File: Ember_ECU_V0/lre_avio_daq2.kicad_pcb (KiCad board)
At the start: 4 copper layers, 13.4 x 4.5 mm, 172 parts, among them J1 Conn_01x02_Socket, J10 Conn_01x02_Pin, J11 USB_C_Receptacle_USB2.0_16P, J12 XT30PW-F, J13 XT30PW-F, J14 XT30PW-F, J15 XT30PW-F, J16 XT30PW-F, J17 SMPW-CC-K-M, J18 SMPW-CC-K-M, J19 SMPW-CC-K-M, J2 DB25_Socket_MountingHoles, J20 Conn_01x02_Pin, J23 DA15_Socket_MountingHoles, J24 DB25_Socket_MountingHoles, J3 XT60PW-M, J4 Conn_01x02_Socket, Q1 SISA96DN-T1-GE3, Q2 SISA96DN-T1-GE3, Q3 SISA96DN-T1-GE3, SW1 SW_SPDT, U1 AMS1117-5.0, U10 ADS8353QPWRQ1, U11 ADS8353QPWRQ1, U12 STM32F412VGTx, U13 HX711, U14 HX711, U15 WS2812B-2020, U16 WS2812B-2020, U17 WS2812B-2020, U18 TCAN330, U2 HX711, U4 HX711, U5 AMS1117-5.0, U6 ADS8353QPWRQ1, U7 MAX31856, U8 MAX31856, U9 MAX31856, Y1 Crystal_8Mhz

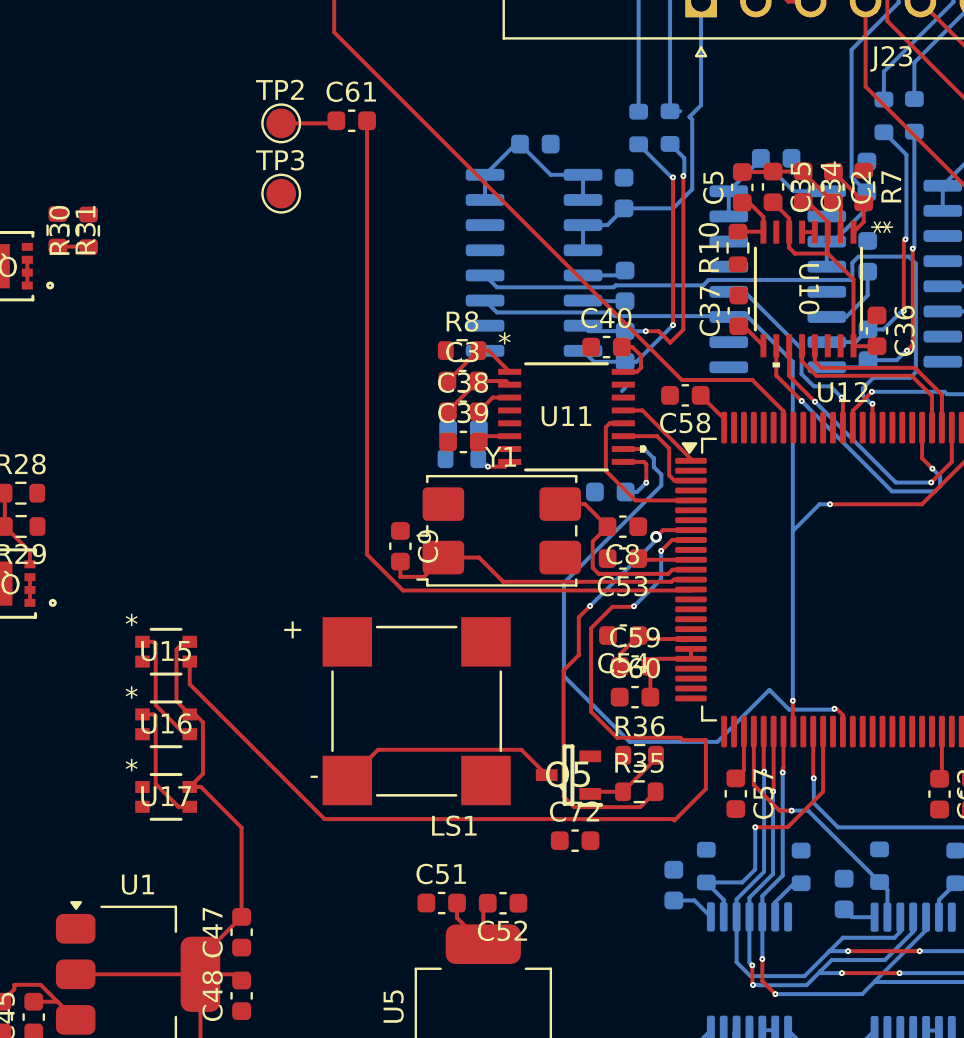
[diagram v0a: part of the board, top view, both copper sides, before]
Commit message: partial schematics fixes
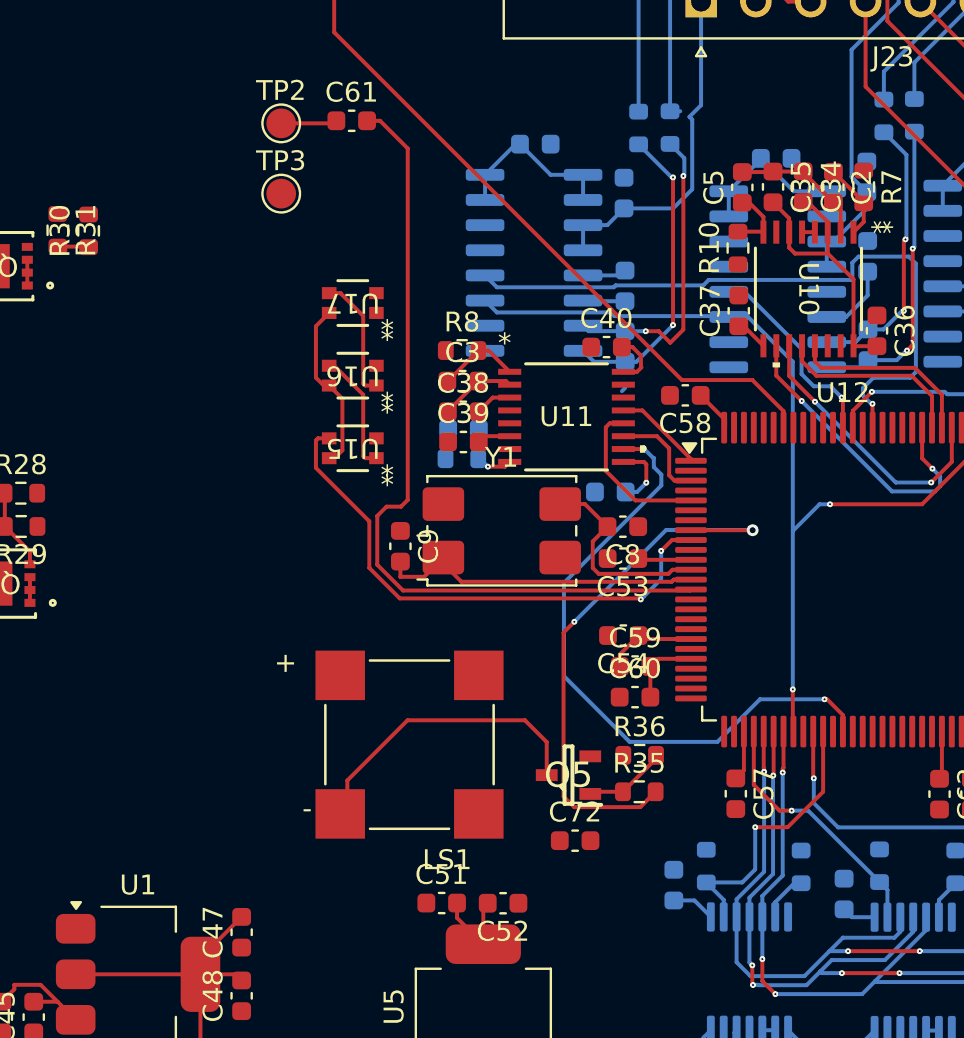
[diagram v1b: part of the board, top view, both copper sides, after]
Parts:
- moved U17 26.7 mm to (189.7, 65.6), turned to 180 degrees
- moved U16 20.0 mm to (189.7, 69.3), turned to 180 degrees
- moved U15 13.9 mm to (189.7, 72.9), turned to 180 degrees
- moved LS1 1.73 mm to (192.5, 87.9)
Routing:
- net /DI1: track 51.5 -> 27.3 mm
- net /5v: track 89.3 -> 81.3 mm
- net /Buzzer_G: track 22.2 -> 28.5 mm
- net Net-(Q5-D): track 11.2 -> 15.4 mm
- net Net-(U12-NRST): track 39.0 -> 41.1 mm
- net GND: track 36.2 -> 35.7 mm

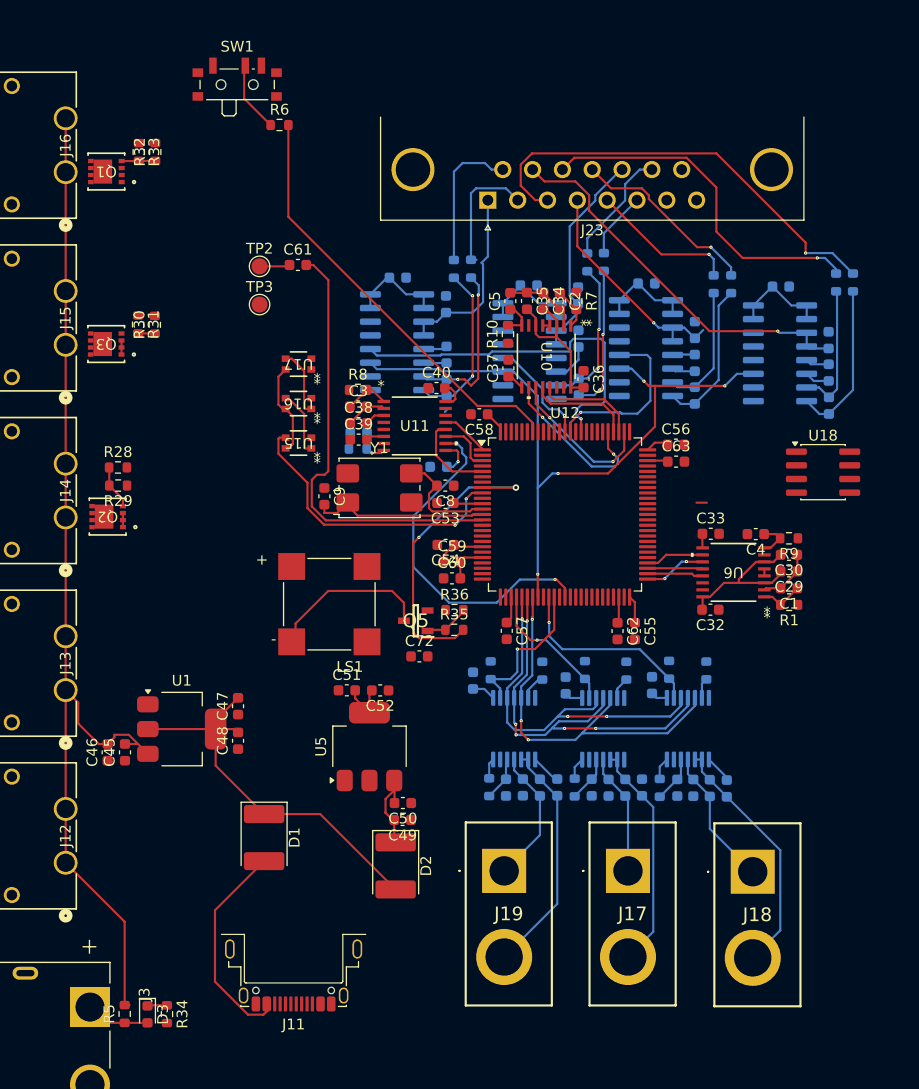
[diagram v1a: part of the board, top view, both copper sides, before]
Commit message: mera last commit till 31/10
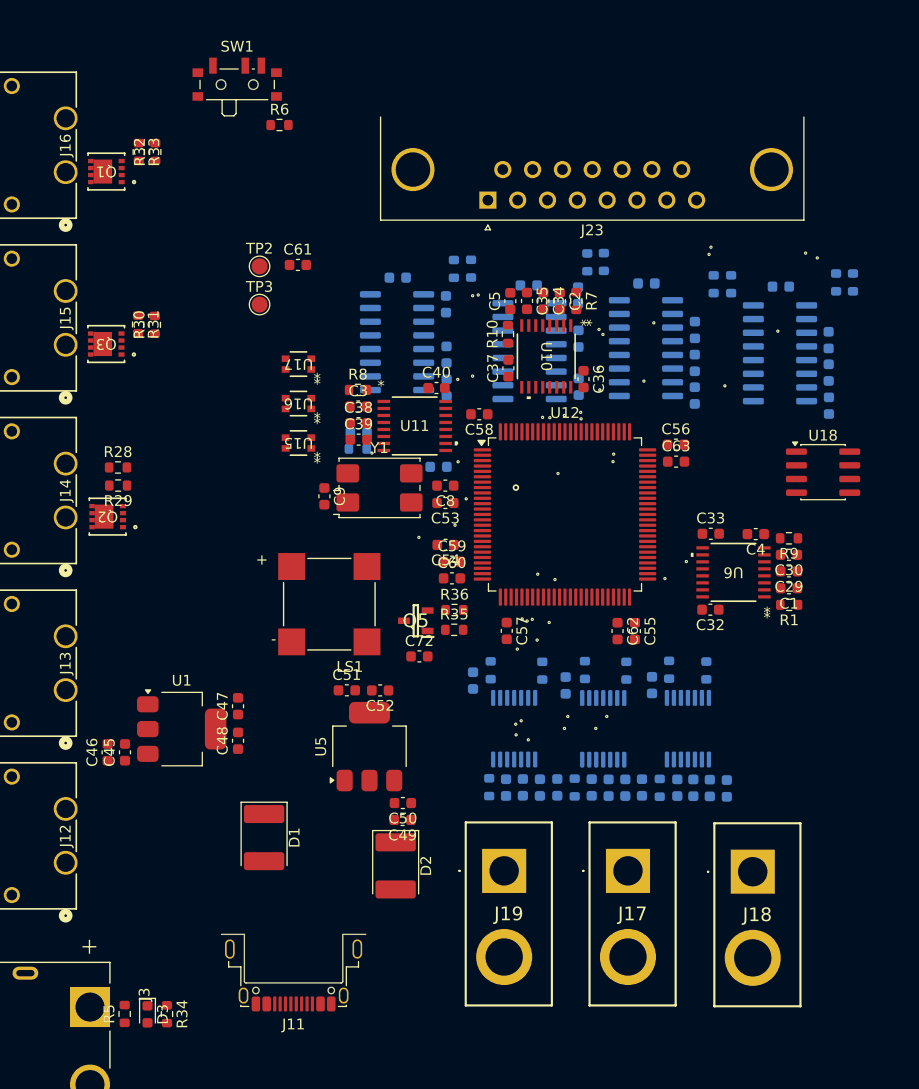
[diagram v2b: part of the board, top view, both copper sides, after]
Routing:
- net /7v4: track 100.0 -> 0.00 mm
- net /3v3: track 81.5 -> 0.00 mm
- net /5v: track 81.3 -> 0.00 mm
- net /HX711_SCK: track 66.1 -> 0.00 mm
- net /S+2: track 41.5 -> 0.00 mm
- net Net-(U12-NRST): track 41.1 -> 0.00 mm
- net Net-(U12-BOOT0): track 40.0 -> 0.00 mm
- net /SPI1_MISO: track 37.5 -> 0.00 mm
- net /E+2: track 36.0 -> 0.00 mm
- net /SPI1_MOSI: track 35.9 -> 0.00 mm
- net GND: track 35.7 -> 0.00 mm
- net /SPI1_SCK: track 35.1 -> 0.00 mm
- net /HX711_DOUT1: track 34.0 -> 0.00 mm
- net /S-2: track 33.0 -> 0.00 mm
- net /SPI4_MOSI: track 32.5 -> 0.00 mm
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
